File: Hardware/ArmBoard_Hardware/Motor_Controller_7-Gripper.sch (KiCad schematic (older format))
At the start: 9 parts, among them Q37 BUK7M6R3-40EX, U9 VNH5019A_E

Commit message: late night with the boy
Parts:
- removed Q37: BUK7M6R3-40EX, Package_TO_SOT_SMD:LFPAK33, symbol Transistor_FET:BUK7M6R3-40EX
- removed R100, R101, R96, R97, R98: 1k, Resistor_SMD:R_0603_1608Metric_Pad0.98x0.95mm_HandSolder, symbol Device:R_Small
- removed R102, R99: 3.3k, Resistor_SMD:R_0603_1608Metric_Pad0.98x0.95mm_HandSolder, symbol Device:R_Small
- removed U9: VNH5019A_E, MRDT_ICs:MultiPowerSO_30, symbol ArmBoard_Hardware-rescue:VNH5019A_E-MRDT_ICs
- added C11: C_Small, Capacitor_SMD:C_0603_1608Metric_Pad1.08x0.95mm_HandSolder, symbol Device:C_Small
- added R58: 20k, Resistor_SMD:R_0603_1608Metric_Pad0.98x0.95mm_HandSolder, symbol Device:R
- added R59, R60: 1k, Resistor_SMD:R_0603_1608Metric_Pad0.98x0.95mm_HandSolder, symbol Device:R_Small
- added U16: LTC6900, Package_TO_SOT_SMD:SOT-23-5_HandSoldering, symbol MRDT_Devices:LTC6900
- added U17: TB67H400AFNG,EL, MRDT_ICs:TB67H400AFNG,EL, symbol MRDT_ICs:TB67H400AFNG,EL
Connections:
- net labels added: +5V
- net labels removed: +3.3V, ENa_7, ENb_7
- wire segments 76 -> 55
- no-connect marks 0 -> 4

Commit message: Fixed Oscillators
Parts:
- C11: value C_Small -> .1uF
- U16: symbol MRDT_Devices:LTC6900 -> ArmBoard_Hardware-rescue:LTC6900-MRDT_Devices
- U17: symbol MRDT_ICs:TB67H400AFNG,EL -> ArmBoard_Hardware-rescue:TB67H400AFNG,EL-MRDT_ICs
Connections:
- net +5V: now also R58.1
- net GND: now also C11.2
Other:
- moved on the sheet: C11
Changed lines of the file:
@@
 Wire Wire Line
 	1395 1525 1400 1525
-Wire Wire Line
-	1395 1375 1395 1525
 $Comp
 L Device:C_Small C?
 U 1 1 6248952B
-P 1395 1275
+P 1275 1275
 AR Path="/63845F20/6248952B" Ref="C?"  Part="1"
 AR Path="/63845F62/6248952B" Ref="C11"  Part="1"
-F 0 "C11" H 1487 1321 50  0000 L CNN
-F 1 "C_Small" H 1487 1230 50  0000 L CNN
-F 2 "Capacitor_SMD:C_0603_1608Metric_Pad1.08x0.95mm_HandSolder" H 1395 1275 50  0001 C CNN
-F 3 "~" H 1395 1275 50  0001 C CNN
-	1    1395 1275
+F 0 "C11" H 1367 1321 50  0000 L CNN
+F 1 ".1uF" H 1367 1230 50  0000 L CNN
+F 2 "Capacitor_SMD:C_0603_1608Metric_Pad1.08x0.95mm_HandSolder" H 1275 1275 50  0001 C CNN
+F 3 "~" H 1275 1275 50  0001 C CNN
+	1    1275 1275
 	1    0    0    -1
 $EndComp
@@
 	2420 1425 2960 1425
 $Comp
-L MRDT_Devices:LTC6900 U?
+L ArmBoard_Hardware-rescue:LTC6900-MRDT_Devices U?
 U 1 1 62489547
 P 2030 1385
 AR Path="/63845F20/62489547" Ref="U?"  Part="1"
 AR Path="/63845F62/62489547" Ref="U16"  Part="1"
+AR Path="/62489547" Ref="U16"  Part="1"
 F 0 "U16" H 2100 1670 50  0000 C CNN
 F 1 "LTC6900" H 2100 1579 50  0000 C CNN
@@
 	3760 4325 3760 4200
 $Comp
-L MRDT_ICs:TB67H400AFNG,EL U?
+L ArmBoard_Hardware-rescue:TB67H400AFNG,EL-MRDT_ICs U?
 U 1 1 62489598
 P 3760 2775
@@
 Text GLabel 2810 3620 0    50   Output ~ 0
 OUTa_7
+Wire Wire Line
+	1275 1375 1275 1425
+Connection ~ 1275 1425
+Wire Wire Line
+	1395 1175 1275 1175
+Wire Wire Line
+	1395 1175 1395 1525
+Connection ~ 1395 1175
 $EndSCHEMATC

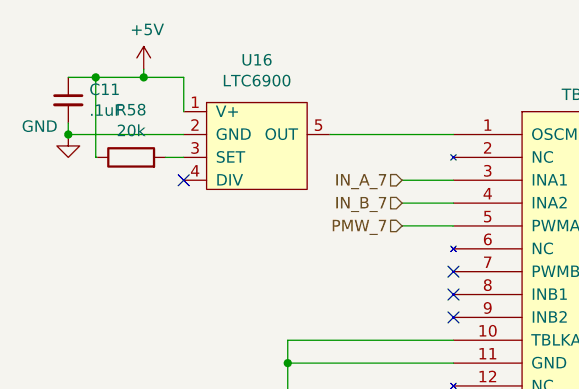
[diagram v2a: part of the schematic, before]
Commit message: armboard review
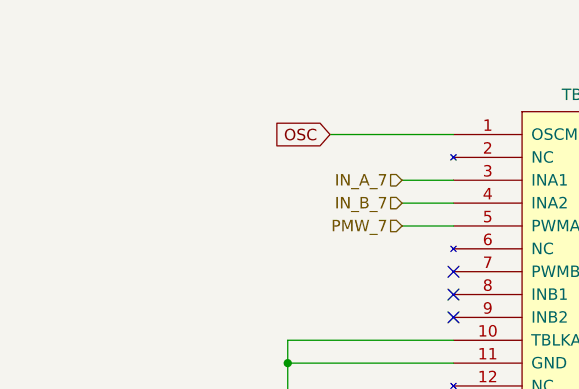
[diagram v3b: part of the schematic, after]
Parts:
- removed C11: .1uF, Capacitor_SMD:C_0603_1608Metric_Pad1.08x0.95mm_HandSolder, symbol Device:C_Small
- removed R58: 20k, Resistor_SMD:R_0603_1608Metric_Pad0.98x0.95mm_HandSolder, symbol Device:R
- removed U16: LTC6900, Package_TO_SOT_SMD:SOT-23-5_HandSoldering, symbol ArmBoard_Hardware-rescue:LTC6900-MRDT_Devices
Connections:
- net OSC: now reaches U17.1 (OSCM)
- no-connect marks 4 -> 3
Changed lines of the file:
@@
 Wire Wire Line
 	2235 2425 2235 2725
-Wire Wire Line
-	1605 1175 1780 1175
-Connection ~ 1605 1175
-Wire Wire Line
-	1605 1175 1605 1140
-Wire Wire Line
-	1395 1175 1605 1175
-Wire Wire Line
-	1780 1175 1780 1325
-$Comp
-L power:+5V #PWR?
-U 1 1 62489523
-P 1605 1140
-AR Path="/63845F20/62489523" Ref="#PWR?"  Part="1"
-AR Path="/63845F62/62489523" Ref="#PWR0107"  Part="1"
-F 0 "#PWR0107" H 1605 990 50  0001 C CNN
-F 1 "+5V" H 1620 1313 50  0000 C CNN
-F 2 "" H 1605 1140 50  0001 C CNN
-F 3 "" H 1605 1140 50  0001 C CNN
-	1    1605 1140
-	1    0    0    -1
-$EndComp
-Wire Wire Line
-	1395 1525 1400 1525
-$Comp
-L Device:C_Small C?
-U 1 1 6248952B
-P 1275 1275
-AR Path="/63845F20/6248952B" Ref="C?"  Part="1"
-AR Path="/63845F62/6248952B" Ref="C11"  Part="1"
-F 0 "C11" H 1367 1321 50  0000 L CNN
-F 1 ".1uF" H 1367 1230 50  0000 L CNN
-F 2 "Capacitor_SMD:C_0603_1608Metric_Pad1.08x0.95mm_HandSolder" H 1275 1275 50  0001 C CNN
-F 3 "~" H 1275 1275 50  0001 C CNN
-	1    1275 1275
-	1    0    0    -1
-$EndComp
-Wire Wire Line
-	1700 1525 1780 1525
-$Comp
-L Device:R R?
-U 1 1 62489532
-P 1550 1525
-AR Path="/63845F20/62489532" Ref="R?"  Part="1"
-AR Path="/63845F62/62489532" Ref="R58"  Part="1"
-F 0 "R58" V 1757 1525 50  0000 C CNN
-F 1 "20k" V 1666 1525 50  0000 C CNN
-F 2 "Resistor_SMD:R_0603_1608Metric_Pad0.98x0.95mm_HandSolder" V 1480 1525 50  0001 C CNN
-F 3 "~" H 1550 1525 50  0001 C CNN
-	1    1550 1525
-	0    -1   -1   0
-$EndComp
-Wire Wire Line
-	1275 1425 1780 1425
-NoConn ~ 1780 1625
-$Comp
-L power:GND #PWR?
-U 1 1 6248953A
-P 1275 1425
-AR Path="/6248953A" Ref="#PWR?"  Part="1"
-AR Path="/62175536/61C88AE8/6248953A" Ref="#PWR?"  Part="1"
-AR Path="/62175536/619EC506/6248953A" Ref="#PWR?"  Part="1"
-AR Path="/6352A127/6248953A" Ref="#PWR?"  Part="1"
-AR Path="/6352A1A0/6248953A" Ref="#PWR?"  Part="1"
-AR Path="/635FA3DE/6248953A" Ref="#PWR?"  Part="1"
-AR Path="/635FA457/6248953A" Ref="#PWR?"  Part="1"
-AR Path="/63845F20/6248953A" Ref="#PWR?"  Part="1"
-AR Path="/63845F62/6248953A" Ref="#PWR0106"  Part="1"
-F 0 "#PWR0106" H 1275 1175 50  0001 C CNN
-F 1 "GND" H 1150 1460 50  0000 C CNN
-F 2 "" H 1275 1425 50  0001 C CNN
-F 3 "" H 1275 1425 50  0001 C CNN
-	1    1275 1425
-	1    0    0    -1
-$EndComp
 $Comp
 L power:+5V #PWR?
@@
 Wire Wire Line
 	2420 1425 2960 1425
-$Comp
-L ArmBoard_Hardware-rescue:LTC6900-MRDT_Devices U?
-U 1 1 62489547
-P 2030 1385
-AR Path="/63845F20/62489547" Ref="U?"  Part="1"
-AR Path="/63845F62/62489547" Ref="U16"  Part="1"
-AR Path="/62489547" Ref="U16"  Part="1"
-F 0 "U16" H 2100 1670 50  0000 C CNN
-F 1 "LTC6900" H 2100 1579 50  0000 C CNN
-F 2 "Package_TO_SOT_SMD:SOT-23-5_HandSoldering" H 2030 1385 50  0001 C CNN
-F 3 "" H 2030 1385 50  0001 C CNN
-	1    2030 1385
-	1    0    0    -1
-$EndComp
 Wire Wire Line
 	2735 1825 2960 1825
@@
 Text GLabel 2810 3620 0    50   Output ~ 0
 OUTa_7
-Wire Wire Line
-	1275 1375 1275 1425
-Connection ~ 1275 1425
-Wire Wire Line
-	1395 1175 1275 1175
-Wire Wire Line
-	1395 1175 1395 1525
-Connection ~ 1395 1175
+Text GLabel 2420 1425 0    50   Input ~ 0
+OSC
 $EndSCHEMATC

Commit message: Rescued the Libaries
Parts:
- U17: symbol ArmBoard_Hardware-rescue:TB67H400AFNG,EL-MRDT_ICs -> MRDT_ICs:TB67H400AFNG,EL
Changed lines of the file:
@@
 	3760 4325 3760 4200
 $Comp
-L ArmBoard_Hardware-rescue:TB67H400AFNG,EL-MRDT_ICs U?
+L MRDT_ICs:TB67H400AFNG,EL U?
 U 1 1 62489598
 P 3760 2775
 AR Path="/63845F20/62489598" Ref="U?"  Part="1"
 AR Path="/63845F62/62489598" Ref="U17"  Part="1"
+AR Path="/62489598" Ref="U17"  Part="1"
 F 0 "U17" H 3760 4390 50  0000 C CNN
 F 1 "TB67H400AFNG,EL" H 3760 4299 50  0000 C CNN
